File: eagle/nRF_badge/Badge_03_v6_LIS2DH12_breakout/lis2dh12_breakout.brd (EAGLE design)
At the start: 11.5 x 13.2 mm, 7 parts, among them U1 LIS2DH12

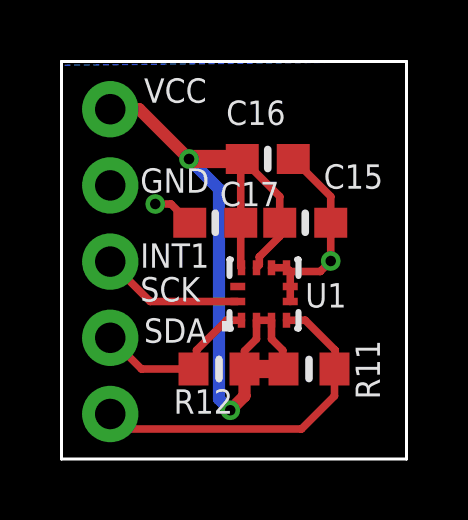
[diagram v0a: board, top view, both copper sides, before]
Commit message: Exporting gerber and pnp
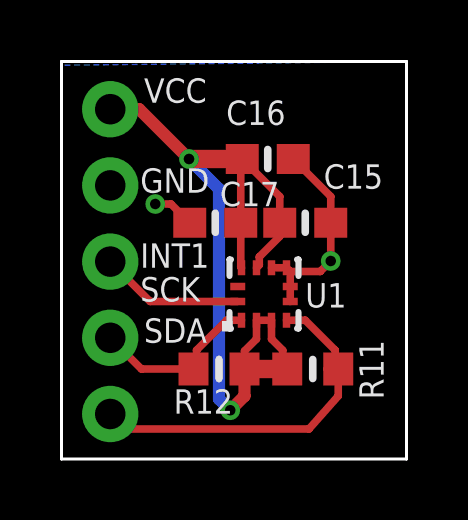
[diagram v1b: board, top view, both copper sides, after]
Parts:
- moved R11 0.12 mm to (8.38, 3.00)
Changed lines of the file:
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@@
 </class>
 </classes>
-<designrules name="PCBNG_DRC_by_oren *">
+<designrules name="PCBNG_DRC_by_oren">
 <description language="de">&lt;b&gt;EAGLE Design Rules&lt;/b&gt;
 &lt;p&gt;
@@
 <param name="mvStopFrame" value="1"/>
 <param name="mvCreamFrame" value="0"/>
-<param name="mlMinStopFrame" value="4mil"/>
+<param name="mlMinStopFrame" value="2mil"/>
 <param name="mlMaxStopFrame" value="4mil"/>
 <param name="mlMinCreamFrame" value="0mil"/>
@@
 <attribute name="NAME" x="7.26" y="9.24" size="0.8128" layer="25" font="vector" ratio="16" rot="R180"/>
 </element>
-<element name="R11" library="rcl" package="R0603" value="1k" x="8.25" y="3" smashed="yes">
-<attribute name="NAME" x="10.615" y="1.99" size="0.8128" layer="25" font="vector" ratio="16" rot="R90"/>
-<attribute name="VALUE" x="7.615" y="0.97" size="0.8128" layer="27" font="vector" ratio="16"/>
+<element name="R11" library="rcl" package="R0603" value="1k" x="8.375" y="3" smashed="yes">
+<attribute name="NAME" x="10.74" y="1.99" size="0.8128" layer="25" font="vector" ratio="16" rot="R90"/>
+<attribute name="VALUE" x="7.74" y="0.97" size="0.8128" layer="27" font="vector" ratio="16"/>
 </element>
 <element name="R12" library="rcl" package="R0603" value="1k" x="5.25" y="3" smashed="yes" rot="R180">
@@
 <wire x1="7" y1="4" x2="7.375" y2="3.625" width="0.254" layer="1"/>
 <wire x1="7.375" y1="3.625" x2="7.375" y2="3.025" width="0.254" layer="1"/>
-<wire x1="7.4" y1="3" x2="7.375" y2="3.025" width="0.254" layer="1"/>
+<wire x1="7.525" y1="3" x2="7.375" y2="3.025" width="0.254" layer="1"/>
 <wire x1="5.975" y1="6.4" x2="5.975" y2="7.875" width="0.254" layer="1"/>
 <wire x1="6" y1="6.375" x2="5.975" y2="6.4" width="0.254" layer="1"/>
@@
 <wire x1="6.025" y1="10" x2="4.25" y2="10" width="0.6096" layer="1"/>
 <via x="5.625" y="1.625" extent="1-16" drill="0.35"/>
-<wire x1="6.1" y1="3" x2="7.4" y2="3" width="0.6096" layer="1"/>
+<wire x1="6.1" y1="3" x2="7.525" y2="3" width="0.6096" layer="1"/>
 <wire x1="4.25" y1="10" x2="5.25" y2="9" width="0.4064" layer="16"/>
 <wire x1="5.25" y1="2" x2="5.625" y2="1.625" width="0.4064" layer="16"/>
@@
 <wire x1="8.125" y1="4.625" x2="9.125" y2="3.625" width="0.254" layer="1"/>
 <wire x1="9.125" y1="3.625" x2="9.125" y2="3.025" width="0.254" layer="1"/>
-<wire x1="9.125" y1="3.025" x2="9.1" y2="3" width="0.254" layer="1"/>
-<wire x1="9.1" y1="3" x2="8.84513125" y2="3" width="0.254" layer="1"/>
-<wire x1="9.1" y1="2.1" x2="9.1" y2="3" width="0.254" layer="1"/>
-<wire x1="9.1" y1="2.1" x2="8" y2="1" width="0.254" layer="1"/>
+<wire x1="9.125" y1="3.025" x2="9.225" y2="3" width="0.254" layer="1"/>
+<wire x1="9.225" y1="3" x2="8.84513125" y2="3" width="0.254" layer="1"/>
+<wire x1="9.225" y1="2.1" x2="9.225" y2="3" width="0.254" layer="1"/>
+<wire x1="9.225" y1="2.1" x2="8.25" y2="1" width="0.254" layer="1"/>
 <contactref element="J2" pad="1"/>
-<wire x1="8" y1="1" x2="2.125" y2="1" width="0.254" layer="1"/>
+<wire x1="8.25" y1="1" x2="2.125" y2="1" width="0.254" layer="1"/>
 <wire x1="2.125" y1="1" x2="1.625" y2="1.5" width="0.254" layer="1"/>
 </signal>
@@
 </signal>
 </signals>
-<errors>
-</errors>
 </board>
 </drawing>
